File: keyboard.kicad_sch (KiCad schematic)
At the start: 46 parts, among them J1 Cirque_GlidePoint, K0 SWITCH_DIODE_1-5U, K1 SWITCH_DIODE_1-5U, K10 SWITCH_DIODE, K11 SWITCH_DIODE, K12 SWITCH_DIODE, K13 SWITCH_DIODE, K14 SWITCH_DIODE, K15 SWITCH_DIODE_2U, K2 SWITCH_DIODE_1-5U, K20 SWITCH_DIODE, K21 SWITCH_DIODE, K22 SWITCH_DIODE, K23 SWITCH_DIODE, K24 SWITCH_DIODE, K25 SWITCH_DIODE, K3 SWITCH_DIODE_1-5U, K30 SWITCH_DIODE, K31 SWITCH_DIODE, K32 SWITCH_DIODE, K33 SWITCH_DIODE, K34 SWITCH_DIODE, K35 SWITCH_DIODE, K4 SWITCH_DIODE, K40 SWITCH_DIODE, K41 SWITCH_DIODE, K42 SWITCH_DIODE, K43 SWITCH_DIODE, K44 SWITCH_DIODE, K45 SWITCH_DIODE, K5 SWITCH_DIODE_2U, K50 SWITCH_DIODE, K51 SWITCH_DIODE, K52 SWITCH_DIODE, K53 SWITCH_DIODE, K55 SWITCH_DIODE, K60 SWITCH_DIODE, K61 SWITCH_DIODE_1-5U, K62 SWITCH_DIODE_1-5U, K63 SWITCH_DIODE, K64 SWITCH_DIODE, K65 SWITCH_DIODE, SW1 evqwdg001, SW2 SW_PUSH, U1 nice_nano

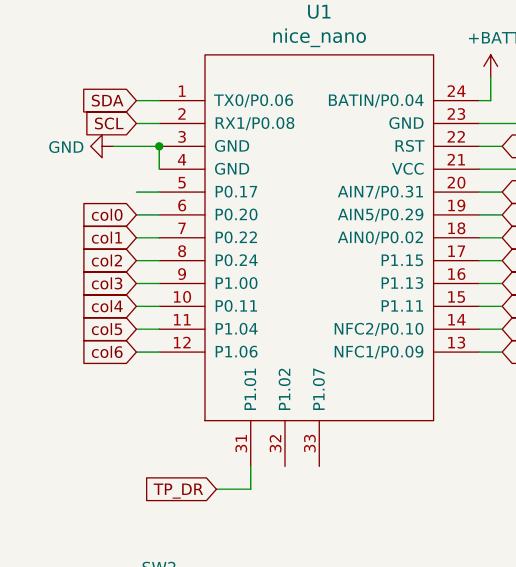
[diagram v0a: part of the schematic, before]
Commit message: readme + routes
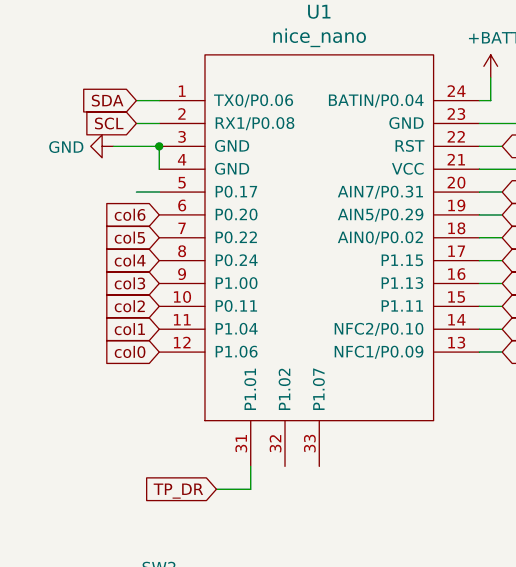
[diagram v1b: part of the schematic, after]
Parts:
- J1: footprint Connector_Hirose:Hirose_DF3EA-12P-2H_1x12-1MP_P2.00mm_Horizontal -> Connector_FFC-FPC:Hirose_FH12-12S-0.5SH_1x12-1MP_P0.50mm_Horizontal
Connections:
- net col0: now also U1.12 (P1.06); no longer U1.6 (P0.20)
- net col1: now also U1.11 (P1.04); no longer U1.7 (P0.22)
- net col2: now also U1.10 (P0.11); no longer U1.8 (P0.24)
- net col4: now also U1.8 (P0.24); no longer U1.10 (P0.11)
- net col5: now also U1.7 (P0.22); no longer U1.11 (P1.04)
- net col6: now also U1.6 (P0.20); no longer U1.12 (P1.06)
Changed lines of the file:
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@@
-    (stroke (width 0) (type default) (color 0 0 0 0))
-  )
-  (wire (pts (xy 25.4 40.64) (xy 27.94 40.64))
     (stroke (width 0) (type default) (color 0 0 0 0))
   )
@@
     (stroke (width 0) (type default) (color 0 0 0 0))
   )
-  (wire (pts (xy 25.4 48.26) (xy 27.94 48.26))
-    (stroke (width 0) (type default) (color 0 0 0 0))
-  )
   (wire (pts (xy 190.5 36.83) (xy 193.04 36.83))
     (stroke (width 0) (type default) (color 0 0 0 0))
@@
     (stroke (width 0) (type default) (color 0 0 0 0))
   )
-  (wire (pts (xy 25.4 50.8) (xy 27.94 50.8))
-    (stroke (width 0) (type default) (color 0 0 0 0))
-  )
   (wire (pts (xy 25.4 35.56) (xy 27.94 35.56))
     (stroke (width 0) (type default) (color 0 0 0 0))
@@
     (stroke (width 0) (type default) (color 0 0 0 0))
   )
-  (wire (pts (xy 25.4 38.1) (xy 27.94 38.1))
-    (stroke (width 0) (type default) (color 0 0 0 0))
-  )
   (wire (pts (xy 132.08 133.35) (xy 132.08 151.13))
     (stroke (width 0) (type default) (color 0 0 0 0))
@@
     (stroke (width 0) (type default) (color 0 0 0 0))
   )
-  (wire (pts (xy 25.4 45.72) (xy 27.94 45.72))
-    (stroke (width 0) (type default) (color 0 0 0 0))
-  )
   (wire (pts (xy 115.57 146.05) (xy 133.35 146.05))
     (stroke (width 0) (type default) (color 0 0 0 0))
@@
     (stroke (width 0) (type default) (color 0 0 0 0))
   )
-  (wire (pts (xy 27.94 53.34) (xy 25.4 53.34))
-    (stroke (width 0) (type default) (color 0 0 0 0))
-  )
   (wire (pts (xy 180.34 67.31) (xy 180.34 52.07))
     (stroke (width 0) (type default) (color 0 0 0 0))
@@
   )
   (wire (pts (xy 66.04 48.26) (xy 63.5 48.26))
-    (stroke (width 0) (type default) (color 0 0 0 0))
-  )
-  (wire (pts (xy 25.4 43.18) (xy 27.94 43.18))
     (stroke (width 0) (type default) (color 0 0 0 0))
   )
@@
     (effects (font (size 1.27 1.27)) (justify left bottom))
   )
-  (global_label "col5" (shape input) (at 25.4 50.8 180) (fields_autoplaced)
-    (effects (font (size 1.27 1.27)) (justify right))
-    (property "Odnośniki między arkuszami" "${INTERSHEET_REFS}" (id 0) (at 0 0 0)
+  (global_label "col5" (shape input) (at 27.94 40.64 180) (fields_autoplaced)
+    (effects (font (size 1.27 1.27)) (justify right))
+    (property "Odnośniki między arkuszami" "${INTERSHEET_REFS}" (id 0) (at 2.54 -10.16 0)
       (effects (font (size 1.27 1.27)) hide)
     )
@@
     )
   )
-  (global_label "col6" (shape input) (at 25.4 53.34 180) (fields_autoplaced)
-    (effects (font (size 1.27 1.27)) (justify right))
-    (property "Odnośniki między arkuszami" "${INTERSHEET_REFS}" (id 0) (at 0 0 0)
+  (global_label "col6" (shape input) (at 27.94 38.1 180) (fields_autoplaced)
+    (effects (font (size 1.27 1.27)) (justify right))
+    (property "Odnośniki między arkuszami" "${INTERSHEET_REFS}" (id 0) (at 2.54 -15.24 0)
       (effects (font (size 1.27 1.27)) hide)
     )
@@
     )
   )
-  (global_label "col2" (shape input) (at 25.4 43.18 180) (fields_autoplaced)
-    (effects (font (size 1.27 1.27)) (justify right))
-    (property "Odnośniki między arkuszami" "${INTERSHEET_REFS}" (id 0) (at 0 0 0)
+  (global_label "col2" (shape input) (at 27.94 48.26 180) (fields_autoplaced)
+    (effects (font (size 1.27 1.27)) (justify right))
+    (property "Odnośniki między arkuszami" "${INTERSHEET_REFS}" (id 0) (at 2.54 5.08 0)
       (effects (font (size 1.27 1.27)) hide)
     )
@@
     )
   )
-  (global_label "col1" (shape input) (at 25.4 40.64 180) (fields_autoplaced)
-    (effects (font (size 1.27 1.27)) (justify right))
-    (property "Odnośniki między arkuszami" "${INTERSHEET_REFS}" (id 0) (at 0 0 0)
+  (global_label "col1" (shape input) (at 27.94 50.8 180) (fields_autoplaced)
+    (effects (font (size 1.27 1.27)) (justify right))
+    (property "Odnośniki między arkuszami" "${INTERSHEET_REFS}" (id 0) (at 2.54 10.16 0)
       (effects (font (size 1.27 1.27)) hide)
     )
@@
     )
   )
-  (global_label "col3" (shape input) (at 25.4 45.72 180) (fields_autoplaced)
-    (effects (font (size 1.27 1.27)) (justify right))
-    (property "Odnośniki między arkuszami" "${INTERSHEET_REFS}" (id 0) (at 0 0 0)
+  (global_label "col3" (shape input) (at 27.94 45.72 180) (fields_autoplaced)
+    (effects (font (size 1.27 1.27)) (justify right))
+    (property "Odnośniki między arkuszami" "${INTERSHEET_REFS}" (id 0) (at 2.54 0 0)
       (effects (font (size 1.27 1.27)) hide)
     )
@@
     )
   )
-  (global_label "col0" (shape input) (at 25.4 38.1 180) (fields_autoplaced)
-    (effects (font (size 1.27 1.27)) (justify right))
-    (property "Odnośniki między arkuszami" "${INTERSHEET_REFS}" (id 0) (at 0 0 0)
+  (global_label "col0" (shape input) (at 27.94 53.34 180) (fields_autoplaced)
+    (effects (font (size 1.27 1.27)) (justify right))
+    (property "Odnośniki między arkuszami" "${INTERSHEET_REFS}" (id 0) (at 2.54 15.24 0)
       (effects (font (size 1.27 1.27)) hide)
     )
@@
     )
   )
-  (global_label "col4" (shape input) (at 25.4 48.26 180) (fields_autoplaced)
-    (effects (font (size 1.27 1.27)) (justify right))
-    (property "Odnośniki między arkuszami" "${INTERSHEET_REFS}" (id 0) (at 0 0 0)
+  (global_label "col4" (shape input) (at 27.94 43.18 180) (fields_autoplaced)
+    (effects (font (size 1.27 1.27)) (justify right))
+    (property "Odnośniki między arkuszami" "${INTERSHEET_REFS}" (id 0) (at 2.54 -5.08 0)
       (effects (font (size 1.27 1.27)) hide)
     )
@@
     (property "Reference" "J1" (id 0) (at 26.67 149.86 0))
     (property "Value" "Cirque_GlidePoint" (id 1) (at 26.67 152.4 0))
-    (property "Footprint" "Connector_Hirose:Hirose_DF3EA-12P-2H_1x12-1MP_P2.00mm_Horizontal" (id 2) (at 30.48 171.45 0)
+    (property "Footprint" "Connector_FFC-FPC:Hirose_FH12-12S-0.5SH_1x12-1MP_P0.50mm_Horizontal" (id 2) (at 30.48 171.45 0)
       (effects (font (size 1.27 1.27)) hide)
     )
@@
     )
     (path "/29682534-0750-4b0d-9c81-581d4025f833"
-      (reference "J1") (unit 1) (value "Cirque_GlidePoint") (footprint "Connector_Hirose:Hirose_DF3EA-12P-2H_1x12-1MP_P2.00mm_Horizontal")
+      (reference "J1") (unit 1) (value "Cirque_GlidePoint") (footprint "Connector_FFC-FPC:Hirose_FH12-12S-0.5SH_1x12-1MP_P0.50mm_Horizontal")
     )
     (path "/aa471460-5937-454e-9ee7-1e2d22862f33"
